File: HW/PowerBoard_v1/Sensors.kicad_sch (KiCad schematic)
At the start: 10 parts, among them U1 MCP9700AT-ETT, U4 AMC130M02DFMR, U5 AMC130M02DFMR

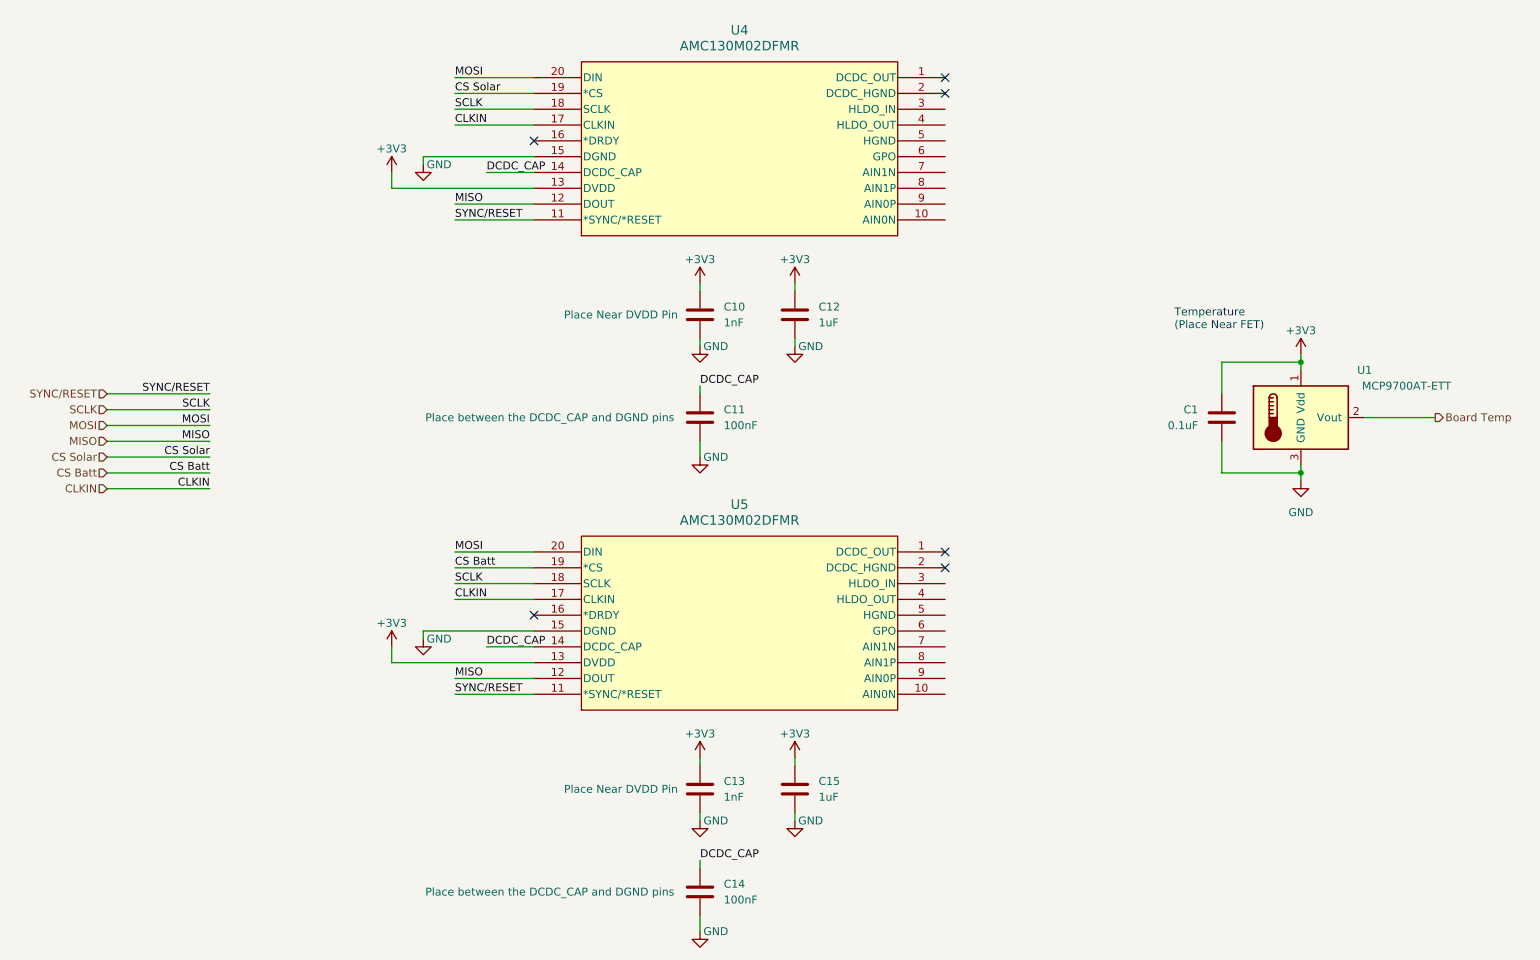
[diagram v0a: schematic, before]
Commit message: updates sensing
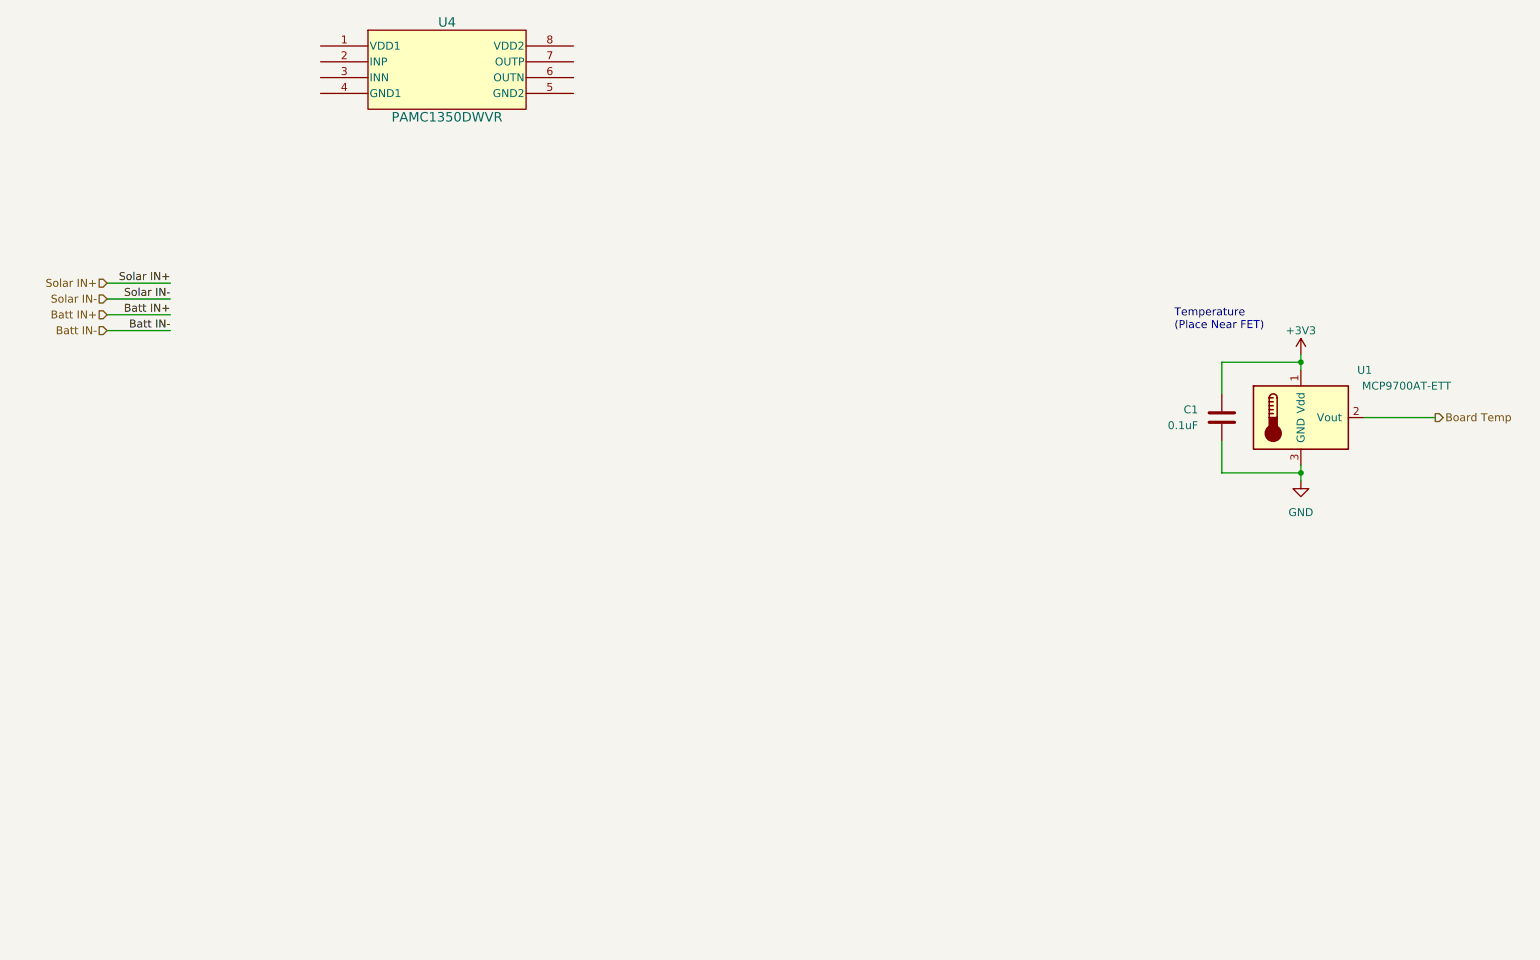
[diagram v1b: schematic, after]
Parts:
- removed C10, C13: 1nF, symbol Device:C
- removed C11, C14: 100nF, symbol Device:C
- removed C12, C15: 1uF, symbol Device:C
- removed U4, U5: AMC130M02DFMR, SOIC20_DFM_TEX, symbol AMC130M02DFMR:AMC130M02DFMR
- added U4: PAMC1350DWVR, U_PAMC1350DWVR_TEX, symbol AMC1350:PAMC1350DWVR
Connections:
- no-connect marks 6 -> 0
